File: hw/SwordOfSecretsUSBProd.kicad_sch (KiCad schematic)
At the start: 14 parts, among them J1 Conn_01x04_Pin, J2 USB_A, J3 Conn_01x04_Pin, J4 Conn_01x04_Pin, SW1 SW_Push, U1 CH340N, U2 AMS1117-3.3, U3 W25Q128JVS, U4 CH32V003F4P6

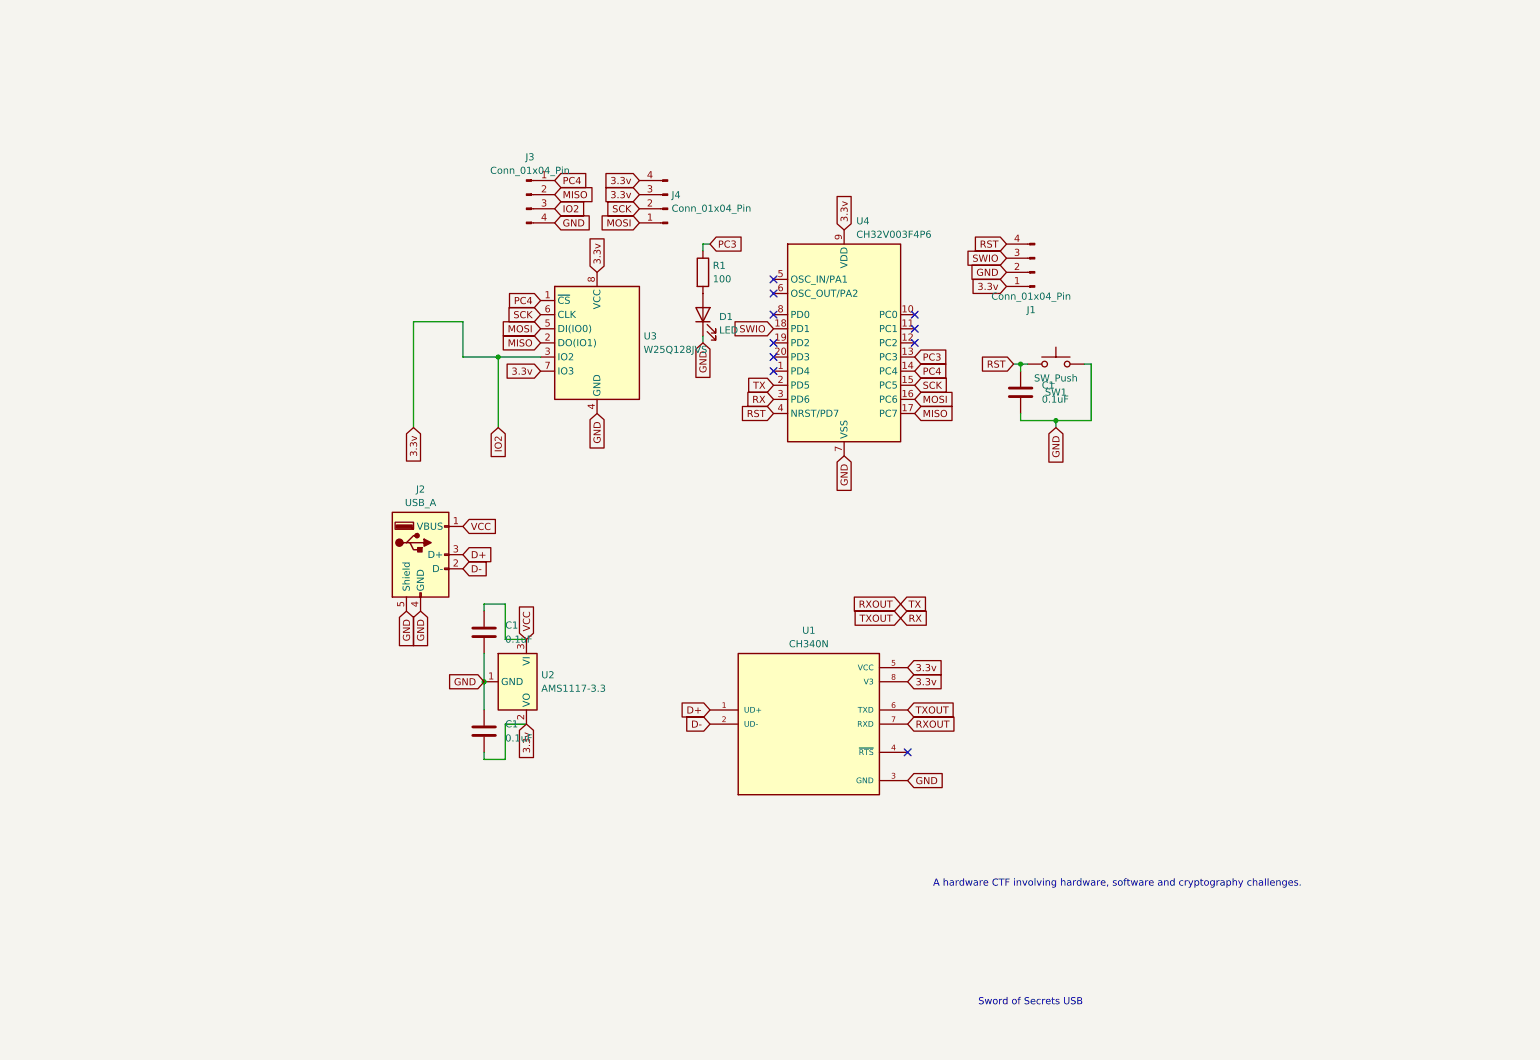
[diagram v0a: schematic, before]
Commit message: chore: Uploading a fancier version of kicad schematics file
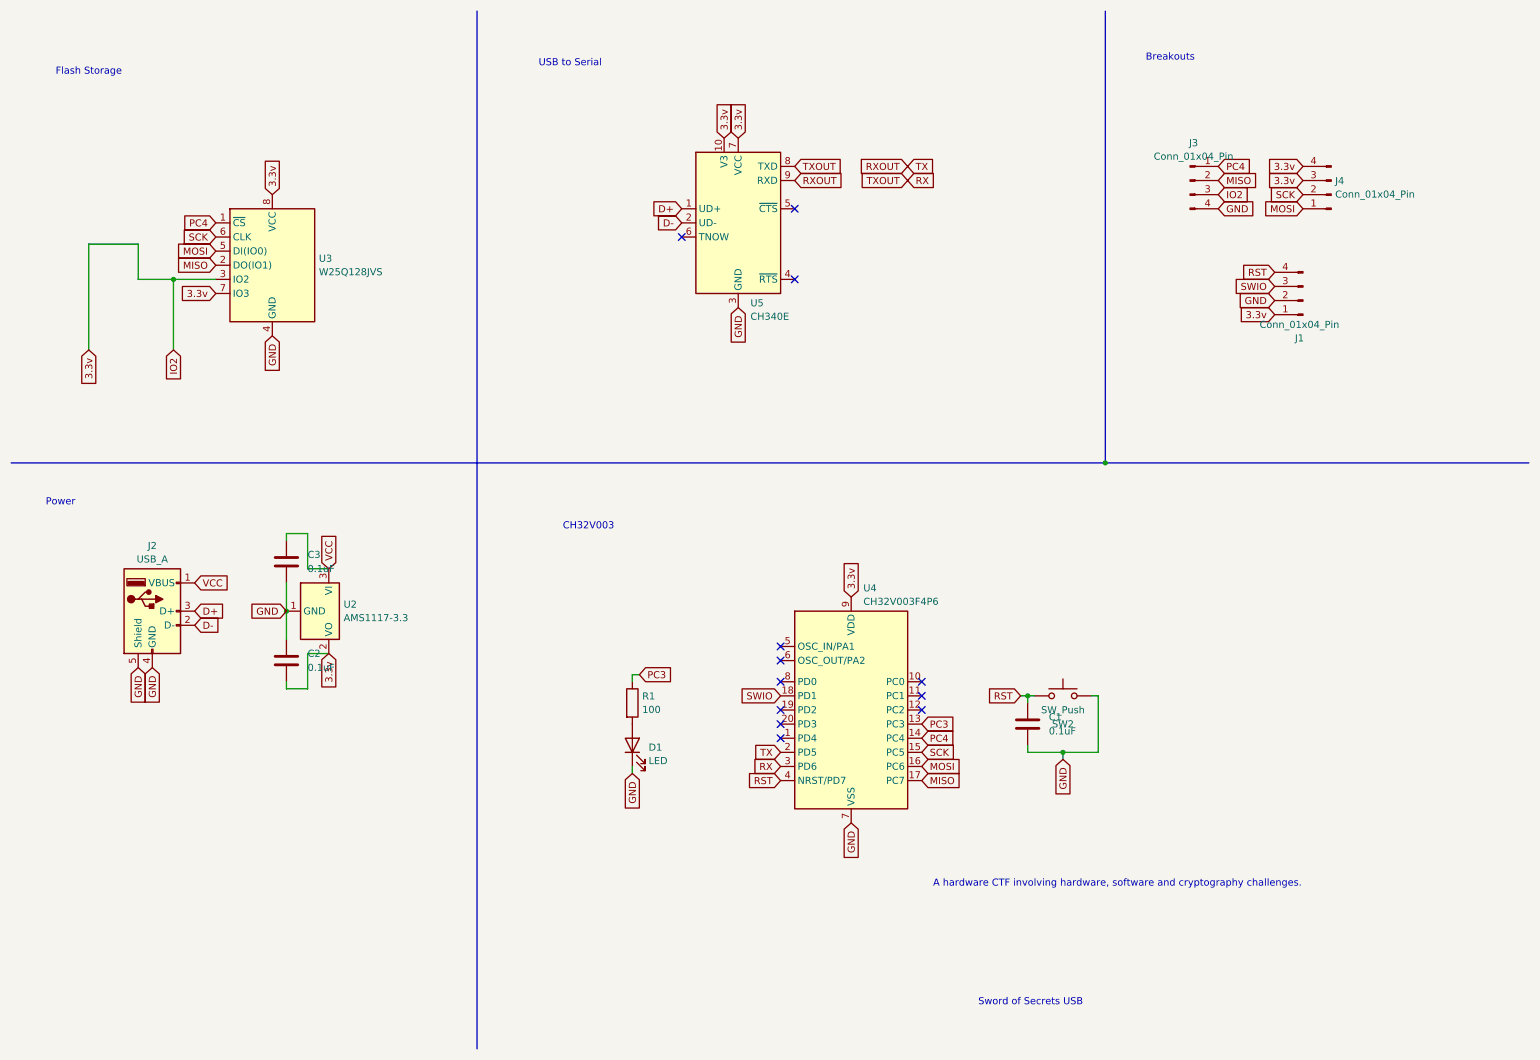
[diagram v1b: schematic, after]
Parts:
- removed U1: CH340N, CH340N:SOIC127P600X160-8N, symbol CH340N:CH340N
- added U5: CH340E, Package_SO:MSOP-10_3x3mm_P0.5mm, symbol Interface_USB:CH340E
- renumbered C1 to C2, C1 to C3, SW1 to SW2
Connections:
- net 3.3v: now also U5.10 (V3), U5.7 (VCC)
- net D+: now also U5.1 (UD+)
- net D-: now also U5.2 (UD-)
- net GND: now also U5.3 (GND)
- net RX: now also U5.8 (TXD)
- net RXOUT: now also U5.9 (RXD)
- no-connect marks 10 -> 12
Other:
- note added: "Breakouts"
- note added: "CH32V003"
- note added: "Flash Storage"
- note added: "Power"
- note added: "USB to Serial"
- moved on the sheet: C1, C2, C3, D1, J1, J2, J3, J4, R1, SW2, U2, U3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
